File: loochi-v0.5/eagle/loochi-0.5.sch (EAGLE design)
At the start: 49 parts, among them IC1 ATTINY61M, J1 SPI_PRG, J2 POWER_JACKSMD, Q1 PMN25ENSOT457, Q2 PMN25ENSOT457, Q3 PMN25ENSOT457, Q4 FDC654P, U1 LZ4-00MC00BIGPADS, U2 APDS-9007, X1 SMA-SMD

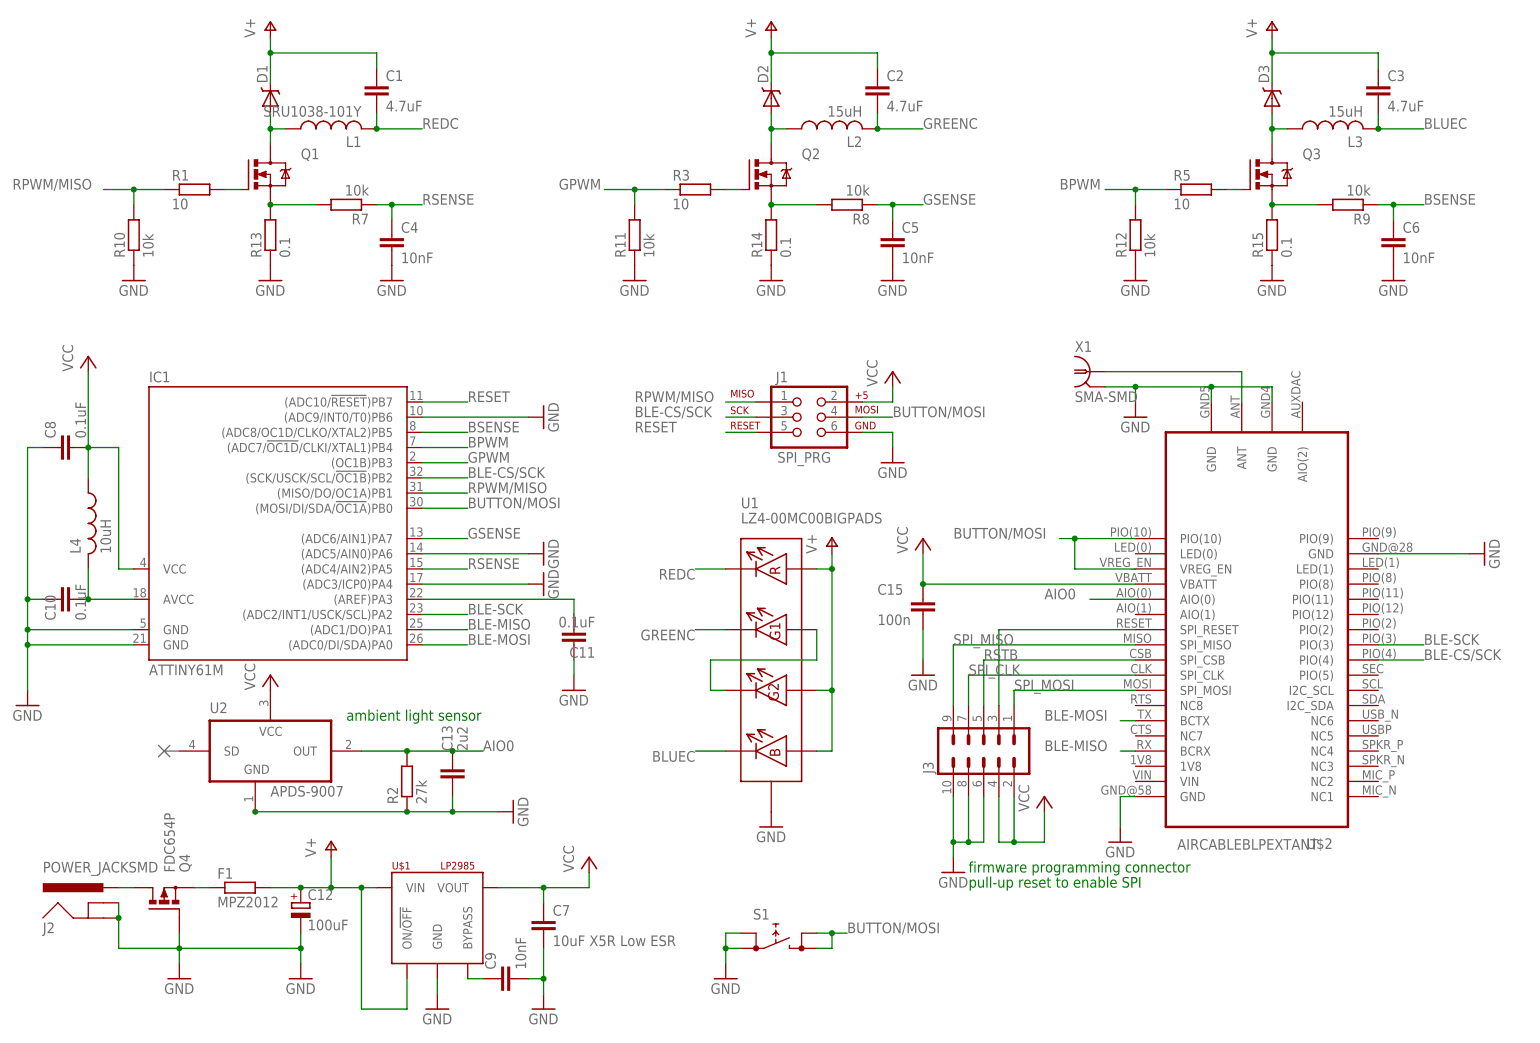
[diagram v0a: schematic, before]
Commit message: loochi-0.5.brd
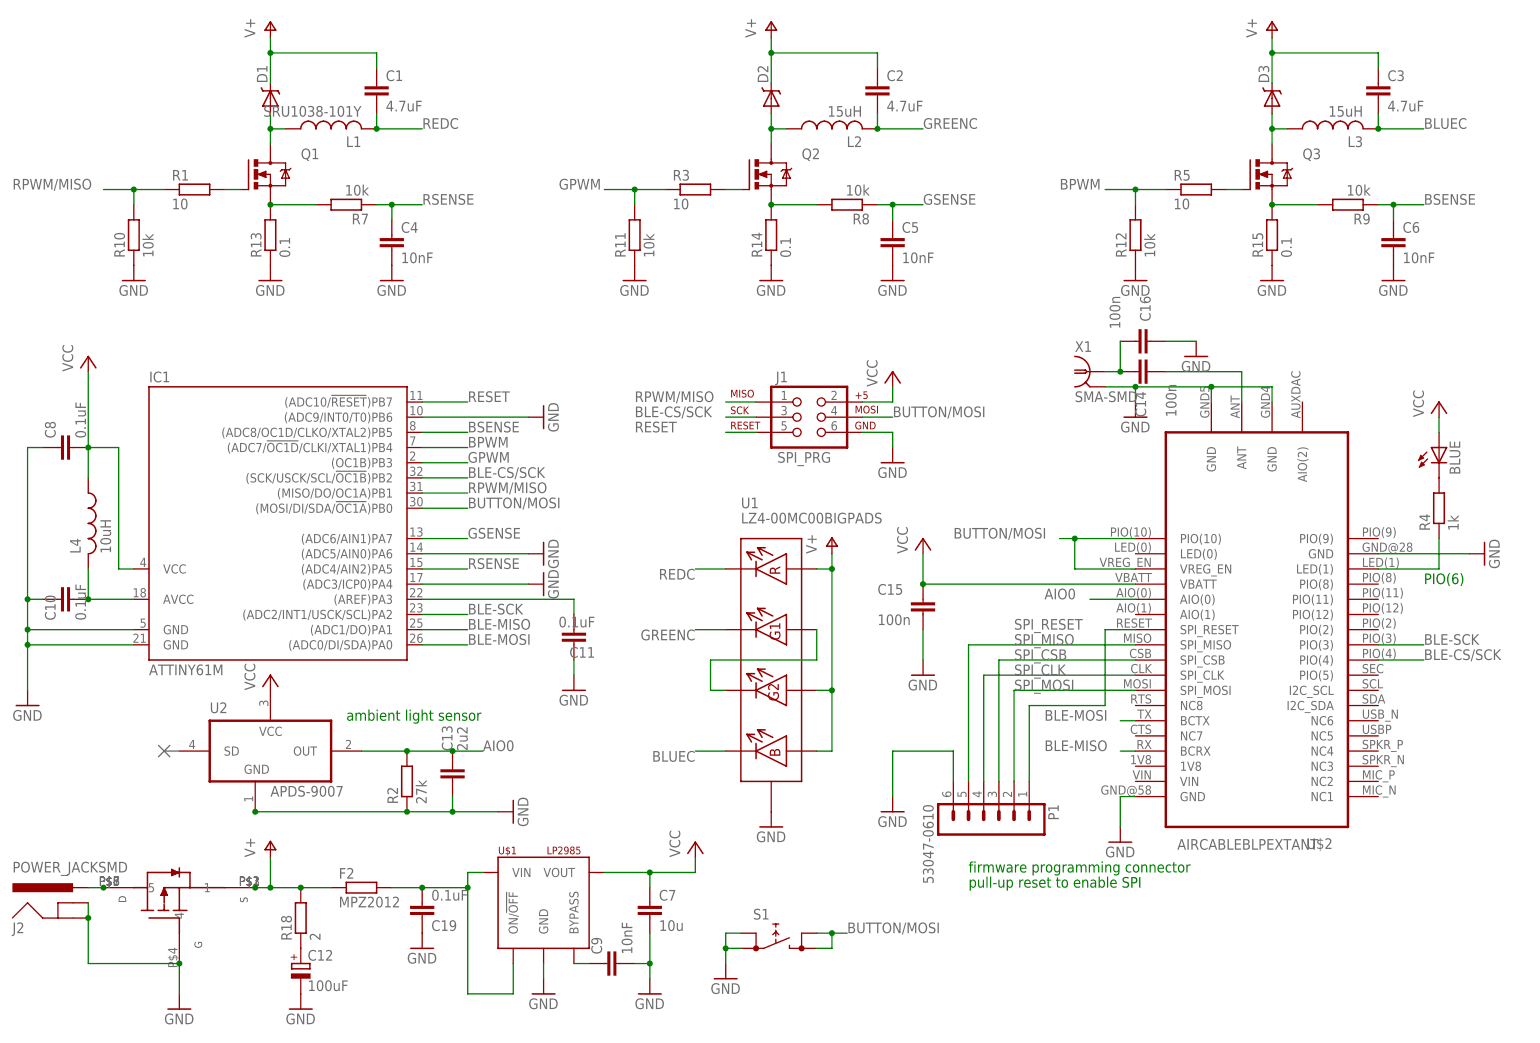
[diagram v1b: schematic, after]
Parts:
- removed F1: MPZ2012, rcl:R-EU_R0603
- removed J3: (no value), con-lstb:MA05-2
- added BLUE: (no value), WCI:500003
- added C14, C16: 100n, rcl:C-EUC0603
- added C19: 0.1uF, rcl:C-EUC0603K
- added F2: MPZ2012, rcl:R-EU_R0603
- added P1: 53047-0610, con-molex-picoblade:53047-0610
- added R18: 2, rcl:R-EU_R0603
- added R4: 1k, rcl:R-EU_R0603
- C7: value 10uF X5R Low ESR -> 10u
- Q4: value FDC654P -> SI7617DN; device mosfet:FDC654P -> Oma:SI7617DN
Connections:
- removed net N$6: F1.1, Q4.S
- removed net RSTB: J3.5, U$2.SPI_CSB
- new net N$12: BLUE.C, R4.2
- new net N$16: R4.1, U$2.LED(1)
- new net N$21: C12.+, R18.1
- new net N$22: C19.2, F2.2, U$1.ON/!OFF!, U$1.VIN
- new net SPI_CSB: P1.3, U$2.SPI_CSB
- new net SPI_RESET: P1.1, U$2.SPI_RESET
- net GND: now also C16.2, C19.1, P1.6, Q4.4; no longer J3.10, J3.6, J3.8, Q4.G
- net N$10: now also Q4.5, Q4.6, Q4.7, Q4.8; no longer Q4.D
- net N$15: now also C14.2, C16.1, X1G$1.1; no longer J3.3, U$2.SPI_RESET
- net N$2: now also C14.1; no longer X1G$1.1
- net SPI_CLK: now also P1.4; no longer J3.7
- net SPI_MISO: now also P1.5; no longer J3.9
- net SPI_MOSI: now also P1.2; no longer J3.1
- net V+: now also F2.1, Q4.1, Q4.2, Q4.3, R18.2; no longer C12.+, F1.2, U$1.ON/!OFF!, U$1.VIN
- net VCC: now also BLUE.A; no longer J3.2, J3.4
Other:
- note added: "PIO(6)"
- moved on the sheet: C12, C7, C9, J2, U$1
